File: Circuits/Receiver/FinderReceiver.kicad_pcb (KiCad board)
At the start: 2 copper layers, 59 x 28 mm, 9 parts, among them P1 WRITER-VCC, SW1 SW_PUSH, U1 TWE_LITE_SMD, U2 NJU72501MJE

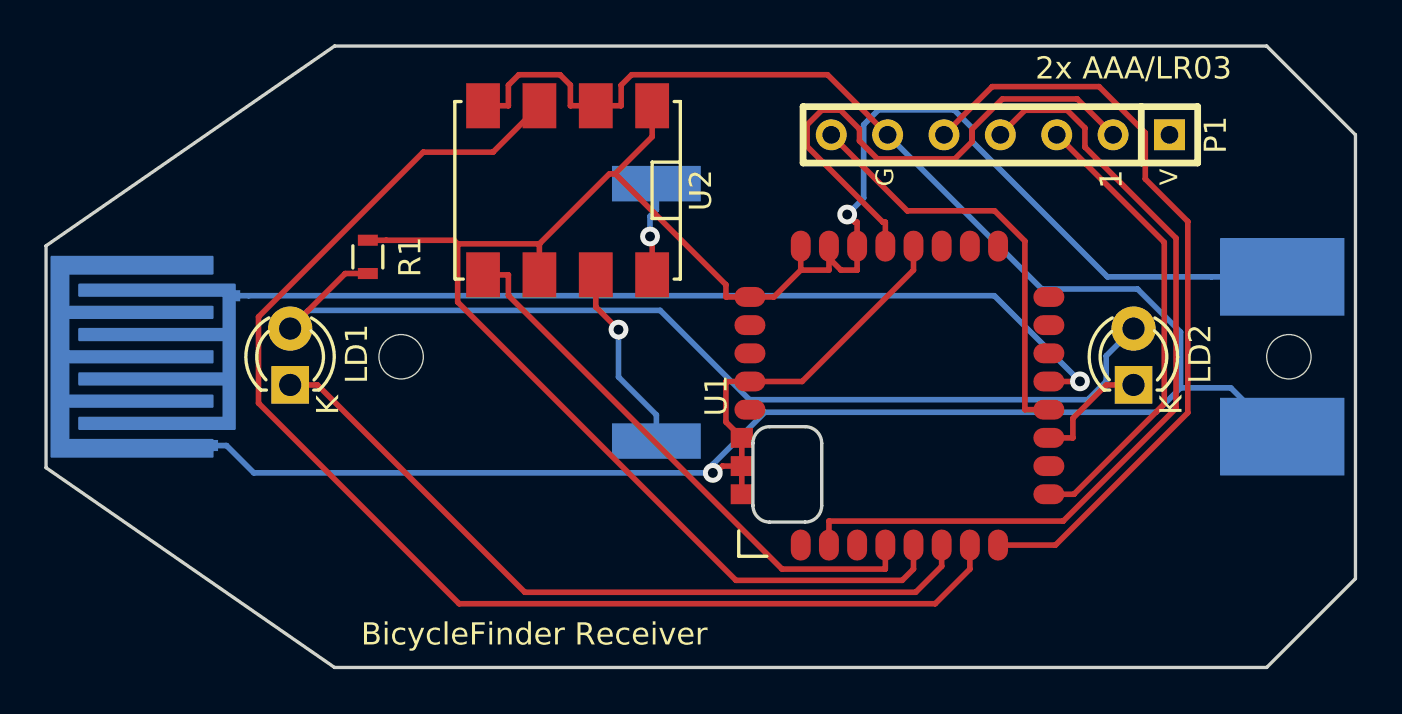
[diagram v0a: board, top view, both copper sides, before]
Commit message: Changed location of parts.
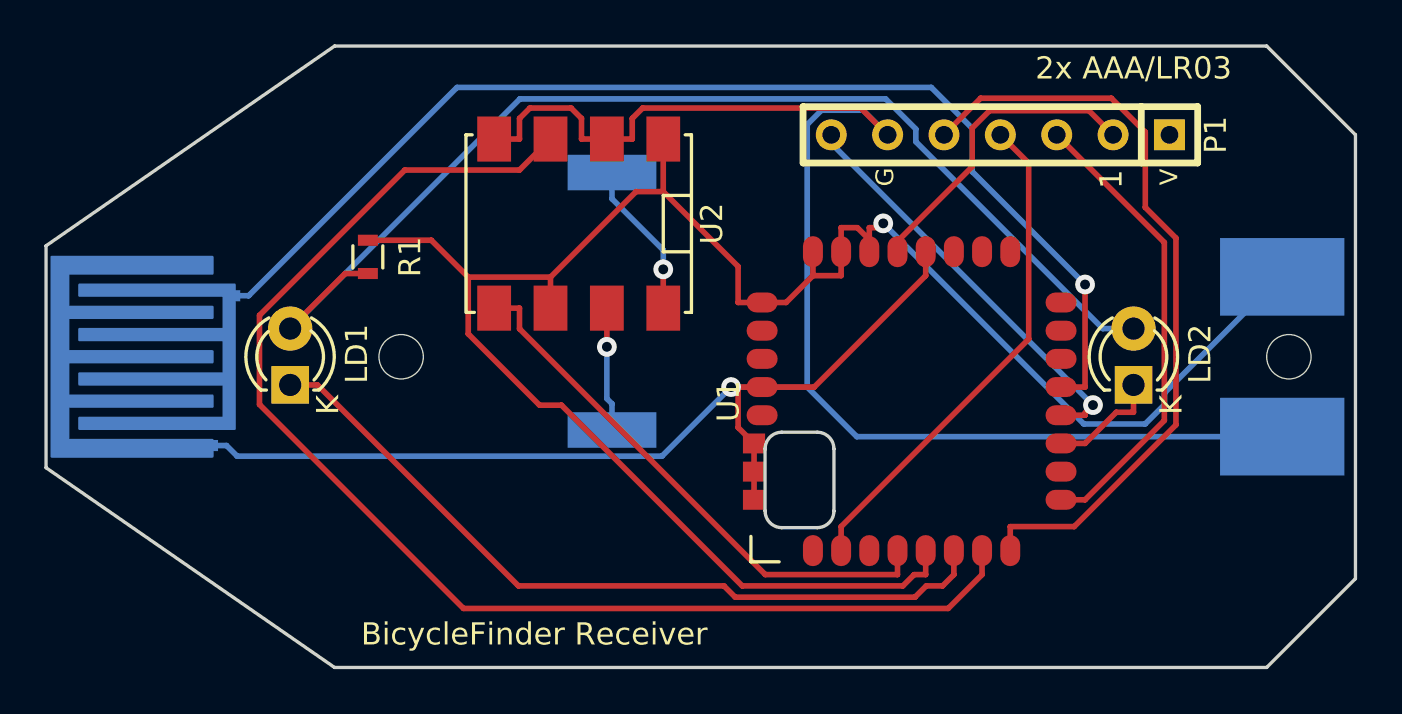
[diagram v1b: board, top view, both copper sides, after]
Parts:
- moved SP1 2.06 mm to (39.5, 27.5)
- moved U2 1.58 mm to (38.0, 24.0)
- moved U1 0.60 mm to (53.0, 32.0)
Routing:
- net /PRG: track 37.8 -> 22.8 mm
- net /DI1: track 41.1 -> 52.7 mm
- net /RST: track 24.4 -> 14.1 mm
- net GND: track 112.0 -> 105.7 mm
- net /LED: track 46.5 -> 51.4 mm
- net /VO2: track 8.62 -> 5.59 mm
- net /VO1: track 4.27 -> 7.07 mm
- net VCC: track 93.5 -> 91.4 mm
- net /DO3: track 34.7 -> 35.4 mm
- net /TXD: track 35.3 -> 34.6 mm
- net /CFG: track 19.4 -> 18.7 mm, vias 0 -> 1
